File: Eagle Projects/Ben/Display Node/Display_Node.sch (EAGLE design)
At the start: 10 parts, among them Q1 16MHz, U1 ATMEGA328P_TQFP

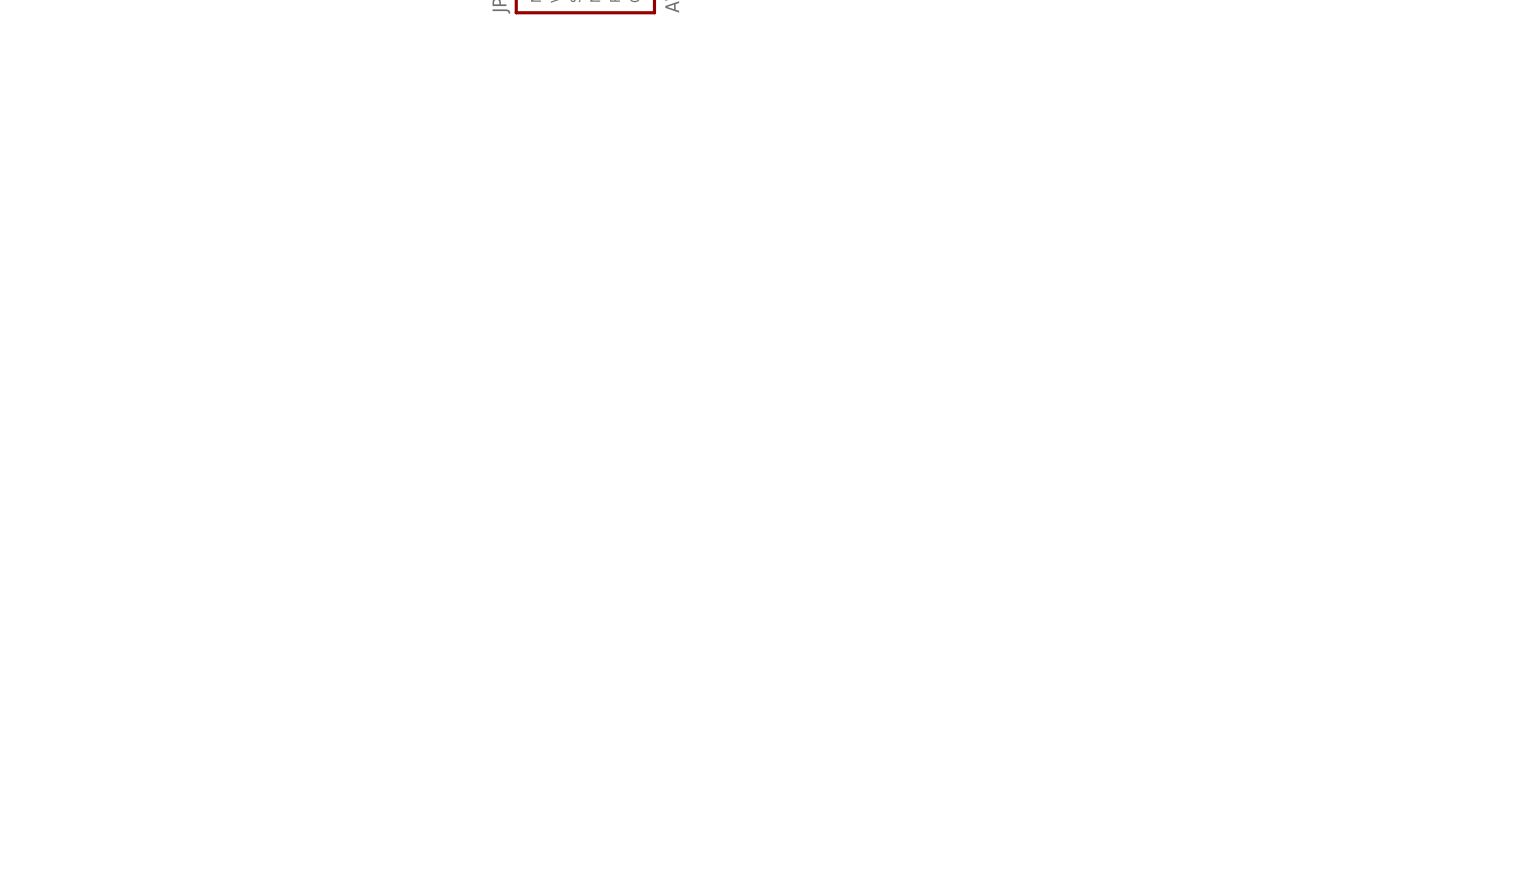
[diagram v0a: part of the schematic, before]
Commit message: Working on PCB's and Generic CAN interface
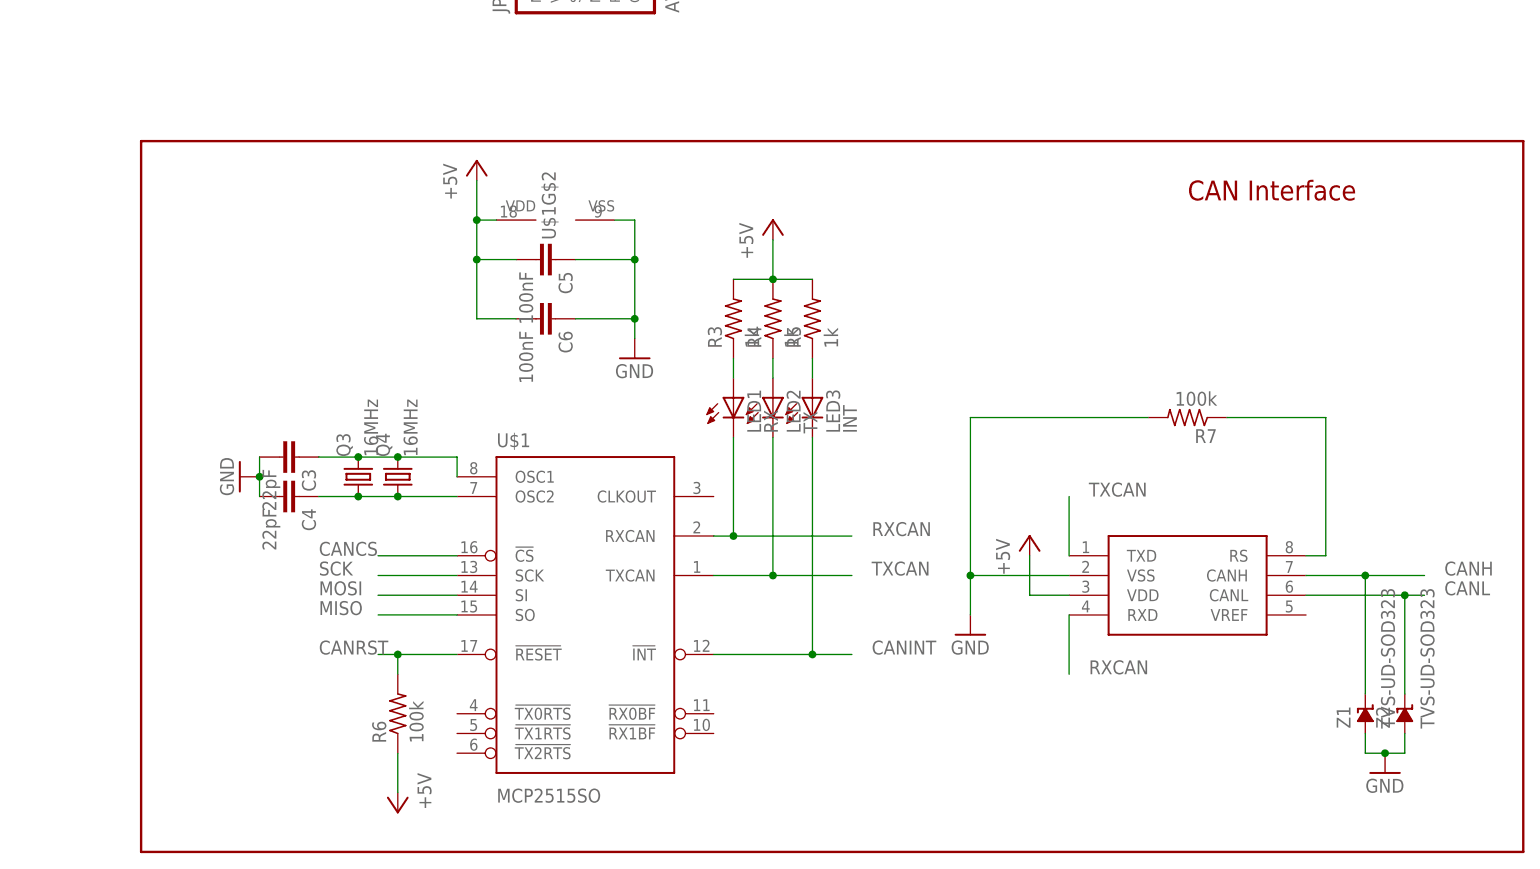
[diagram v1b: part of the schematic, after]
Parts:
- added C3, C4: 22pF, resistor:C-EUC0805K
- added C5, C6: 100nF, resistor:C-EUC0805K
- added LED1: RX, led:LEDCHIP-LED0805
- added LED2: TX, led:LEDCHIP-LED0805
- added LED3: INT, led:LEDCHIP-LED0805
- added Q3: 16MHz, crystal:CRYSTALHC49S
- added Q4: 16MHz, crystal:CRYSTALHC49UP
- added R3, R4, R5: 1k, resistor:R-US_R0805
- added R6, R7: 100k, resistor:R-US_R0805
- added U$1: MCP2515SO, RobThePyro:MCP2515SO
- added U2: MCP2551, SparkFun:MCP2551
- added Z1, Z2: TVS-UD-SOD323, supressor:TVS-UD-SOD323
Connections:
- new net CANCS: U$1G$1.!CS
- new net CANH: U2.CANH, Z1.C
- new net CANINT: LED3.C, U$1G$1.!INT
- new net CANL: U2.CANL, Z2.C
- new net CANRST: R6.2, U$1G$1.!RESET
- new net CANSTBY: R7.1, U2.RS
- new net N$3: C3.1, Q3.2, Q4.2, U$1G$1.OSC1
- new net N$6: C4.1, Q3.1, Q4.1, U$1G$1.OSC2
- new net N$7: LED1.A, R3.1
- new net N$8: LED2.A, R4.1
- new net N$9: LED3.A, R5.1
- new net RXCAN: LED1.C, U$1G$1.RXCAN, U2.RXD
- new net TXCAN: LED2.C, U$1G$1.TXCAN, U2.TXD
- net +5V: now also C5.2, C6.2, R3.2, R4.2, R5.2, R6.1, U$1G$2.VDD, U2.VDD
- net GND: now also C3.2, C4.2, C5.1, C6.1, R7.2, U$1G$2.VSS, U2.VSS, Z1.A, Z2.A
- net MISO: now also U$1G$1.SO
- net MOSI: now also U$1G$1.SI
- net SCK: now also U$1G$1.SCK
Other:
- note added: "CAN Interface"
